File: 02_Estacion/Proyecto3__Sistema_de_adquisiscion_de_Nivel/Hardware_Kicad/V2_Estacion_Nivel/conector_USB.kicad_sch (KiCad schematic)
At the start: 4 parts, among them J9 USB_C_Receptacle_USB2.0_16P

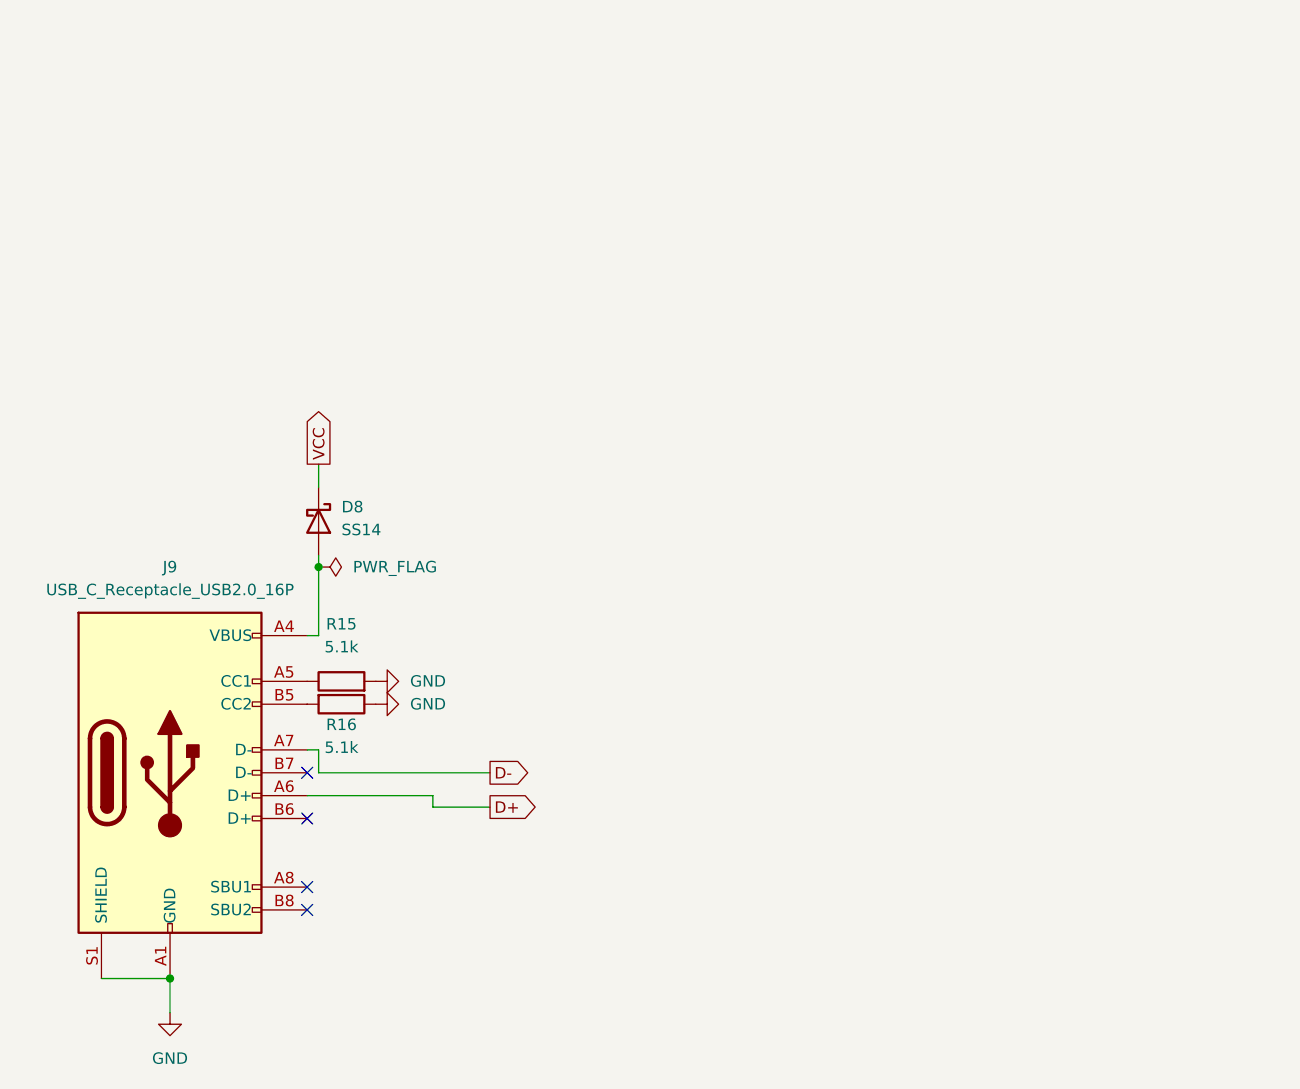
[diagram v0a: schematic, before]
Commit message: update
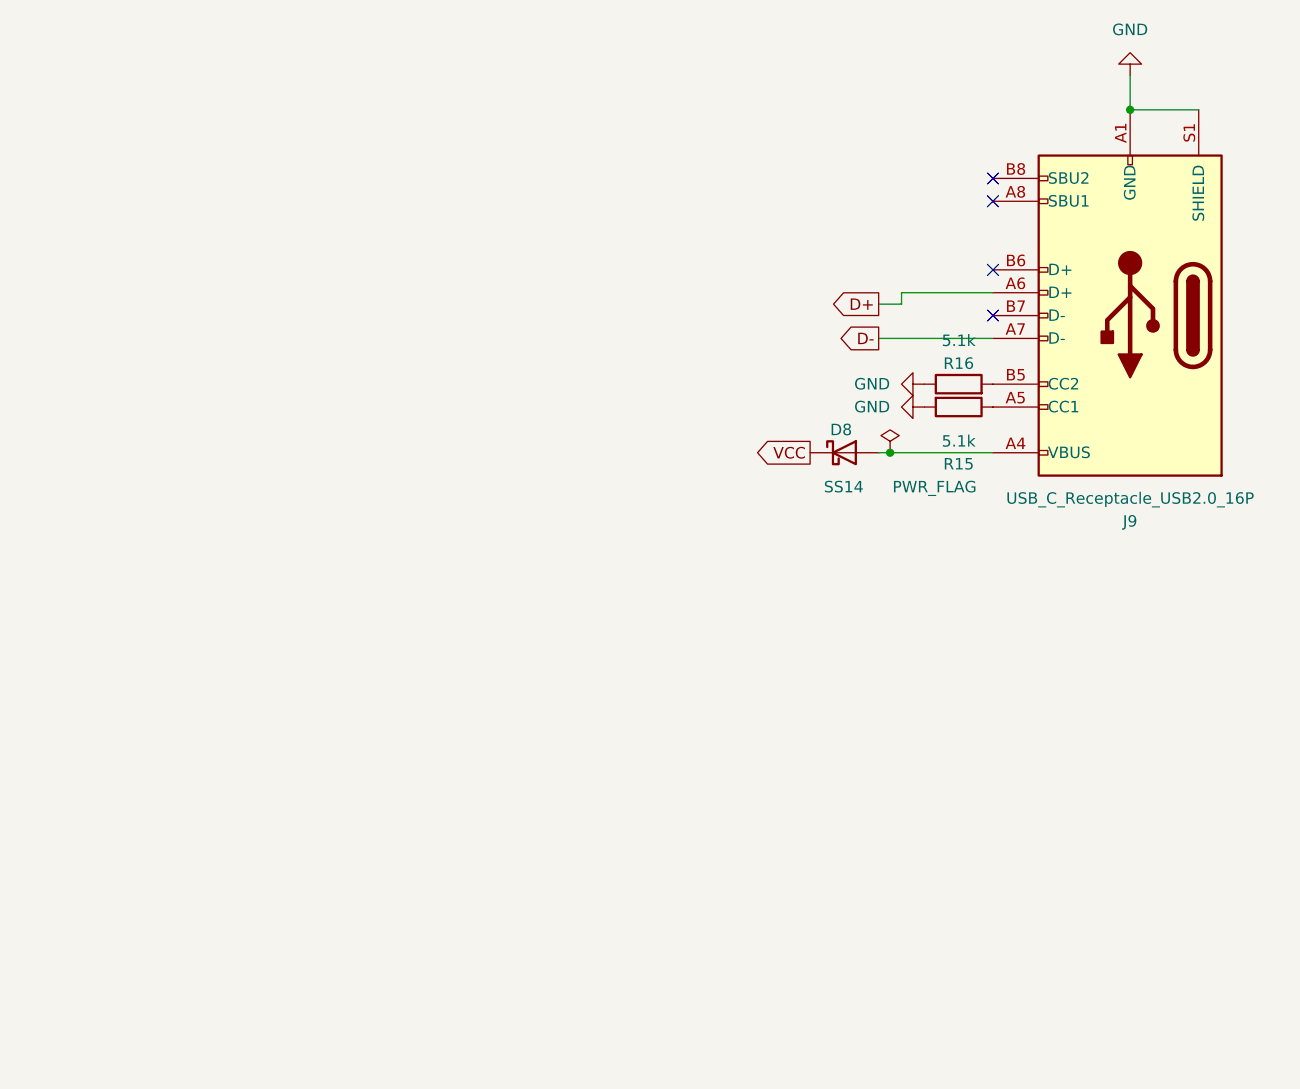
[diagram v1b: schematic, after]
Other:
- moved on the sheet: D8, J9, R15, R16
